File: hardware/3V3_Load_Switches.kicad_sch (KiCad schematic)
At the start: 28 parts, among them Q18 SI2302DDS-T1-GE3, Q19 SI2302DDS-T1-GE3, Q20 SI2302DDS-T1-GE3, U1 LMV321RIYLT, U2 INA199C3DCKR, U3 INA199C3DCKR, U4 INA199C1DCKR, U5 NVTFS5116PLTAG, U6 NVTFS5116PLTAG, U7 NVTFS5116PLTAG

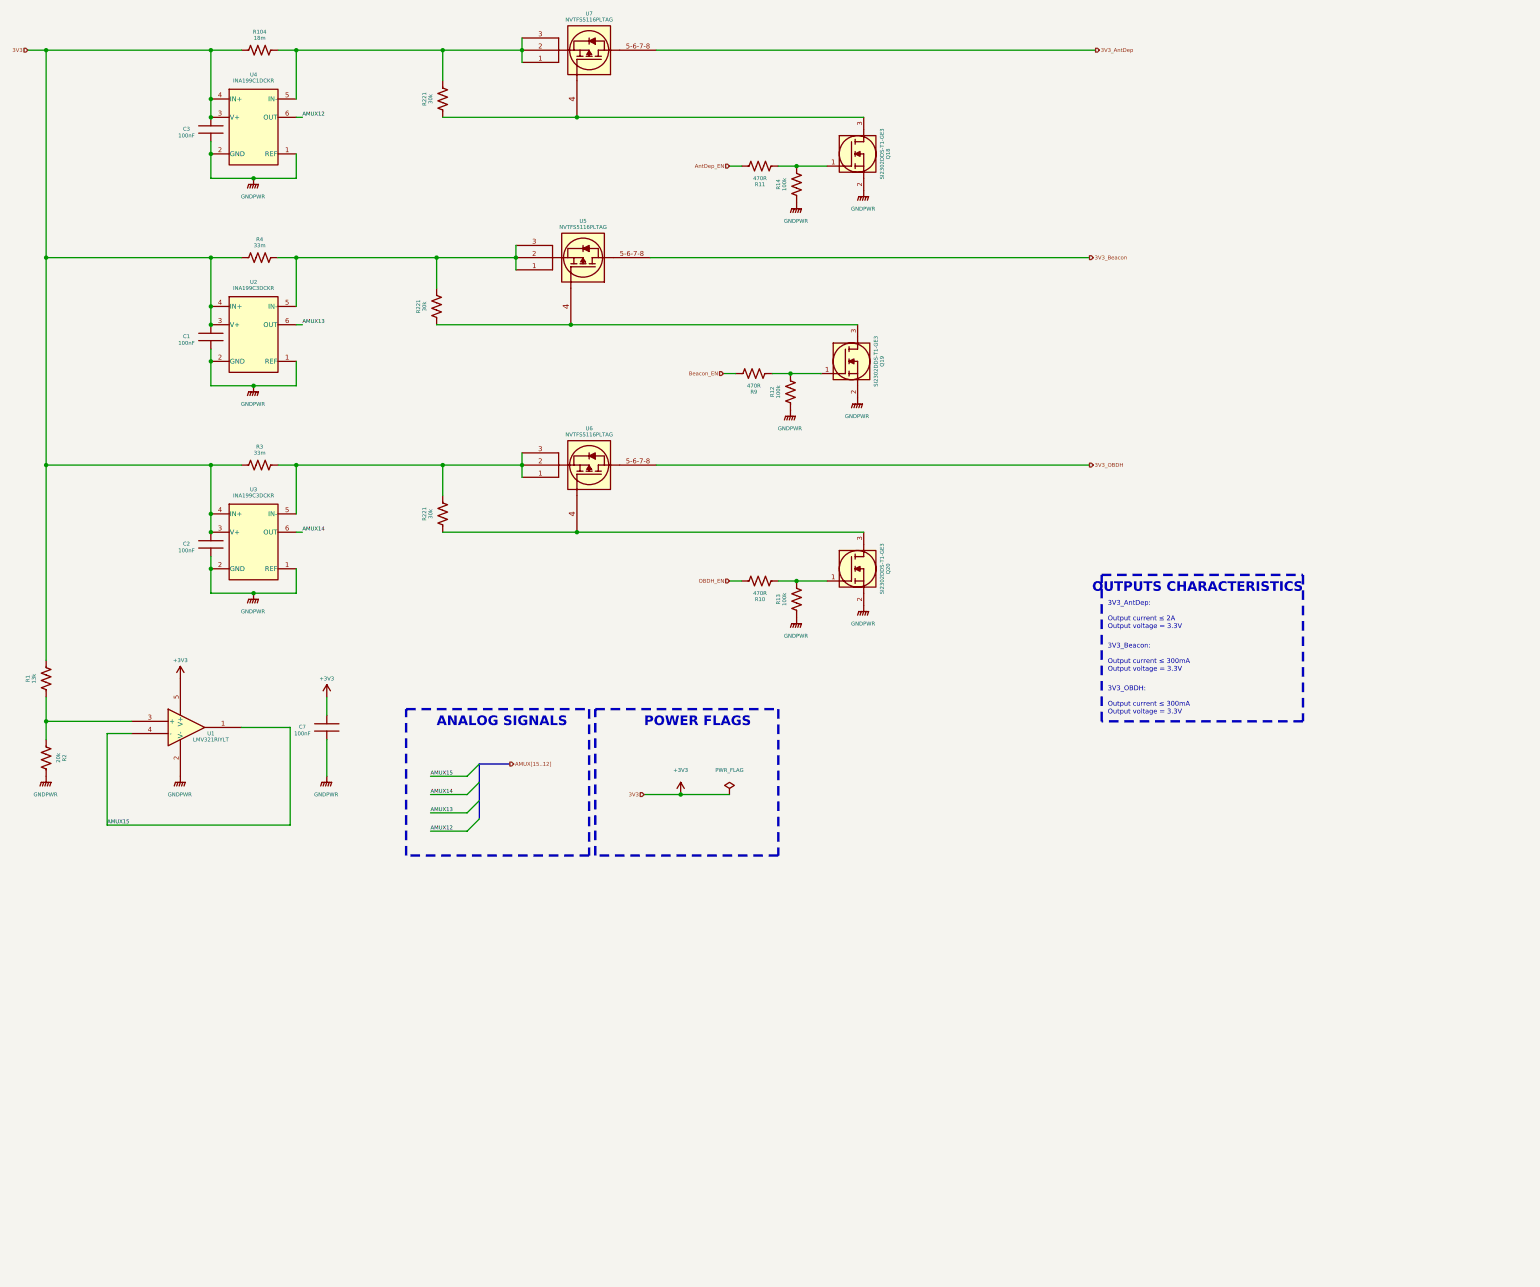
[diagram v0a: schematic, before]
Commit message: hardware: update schematic and layout projects
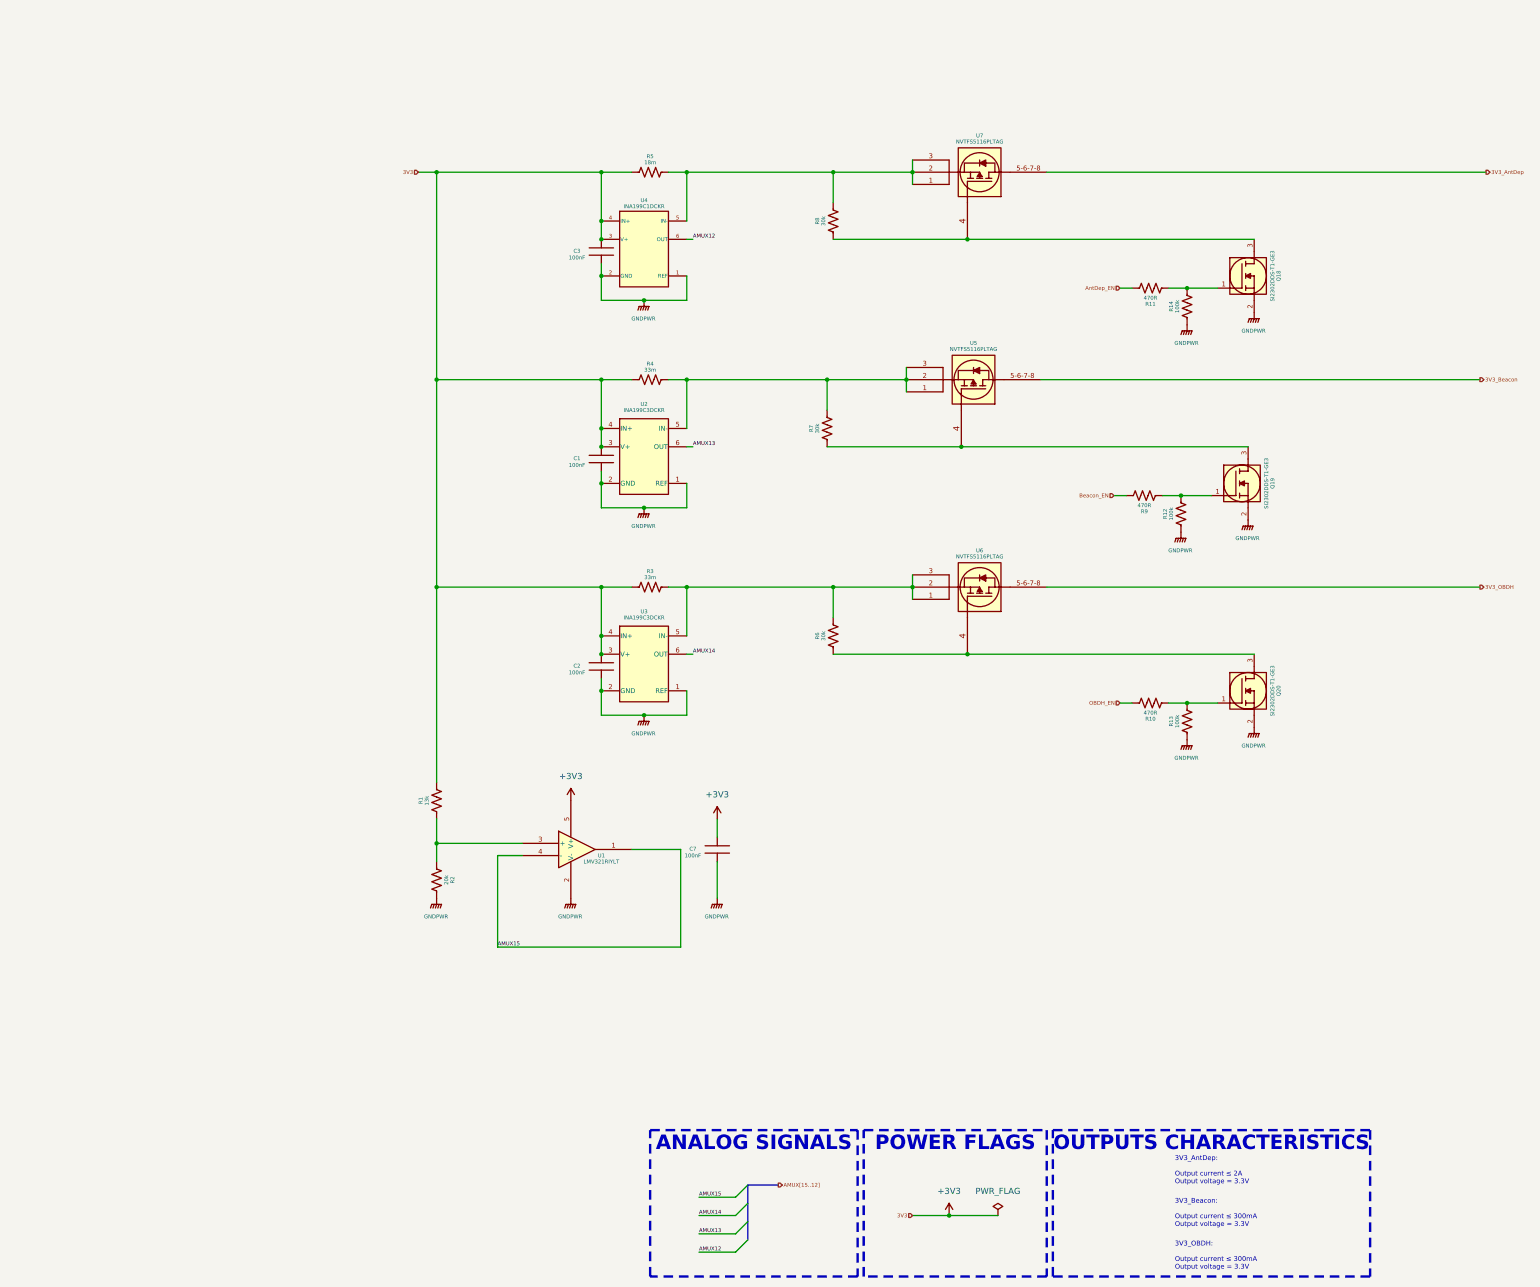
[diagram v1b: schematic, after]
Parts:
- R6, R7, R8: renamed from R221; symbol CRCW060330K0FKEAHP:RES -> CRCW060330K0FKEAHP:CRCW060330K0FKEAHP
- U4: Manufacturer TI -> Texas Instruments
- renumbered R104 to R5
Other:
- note removed: "ANALOG SIGNALS"
- note removed: "OUTPUTS CHARACTERISTICS"
- note removed: "POWER FLAGS"
- moved on the sheet: C1, C2, C3, C7, Q18, Q19, Q20, R1, R10, R11, R12, R13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
